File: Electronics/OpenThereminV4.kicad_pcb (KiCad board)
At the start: 2 copper layers, 50.5 x 127.5 mm, 102 parts, among them J1 USB_C_Receptacle, J2 Conn_02x03_Odd_Even, P1 10k, P10 BUTTON, P11 A3_PAD, P12 A2_PAD, P13 A1_PAD, P14 A0_PAD, P15 CV2, P16 GND, P2 10k, P3 10k, P4 10k, P5 RXD, P6 audio, P7 CV1, P8 VCC, P9 GND, U1 TTP223, U10 FT232RL, U11 LP2985-3.3, U12 MCP4922-E/SL, U2 74HC4060D, U3 74HC4060D, U4 74HC74, U5 HEF4069UBT, U6 MCP4922-E/SL, U7 MCP4922-E/SL, U8 LM358 / MCP6002, U9 ATmega328P-AU, X1 16MHz, X2 7.3721MHz, Y1 MountPad3, Y2 MountPad3, Y3 SJ-3524-SMT-TR, Y7 SJ-3524-SMT-TR

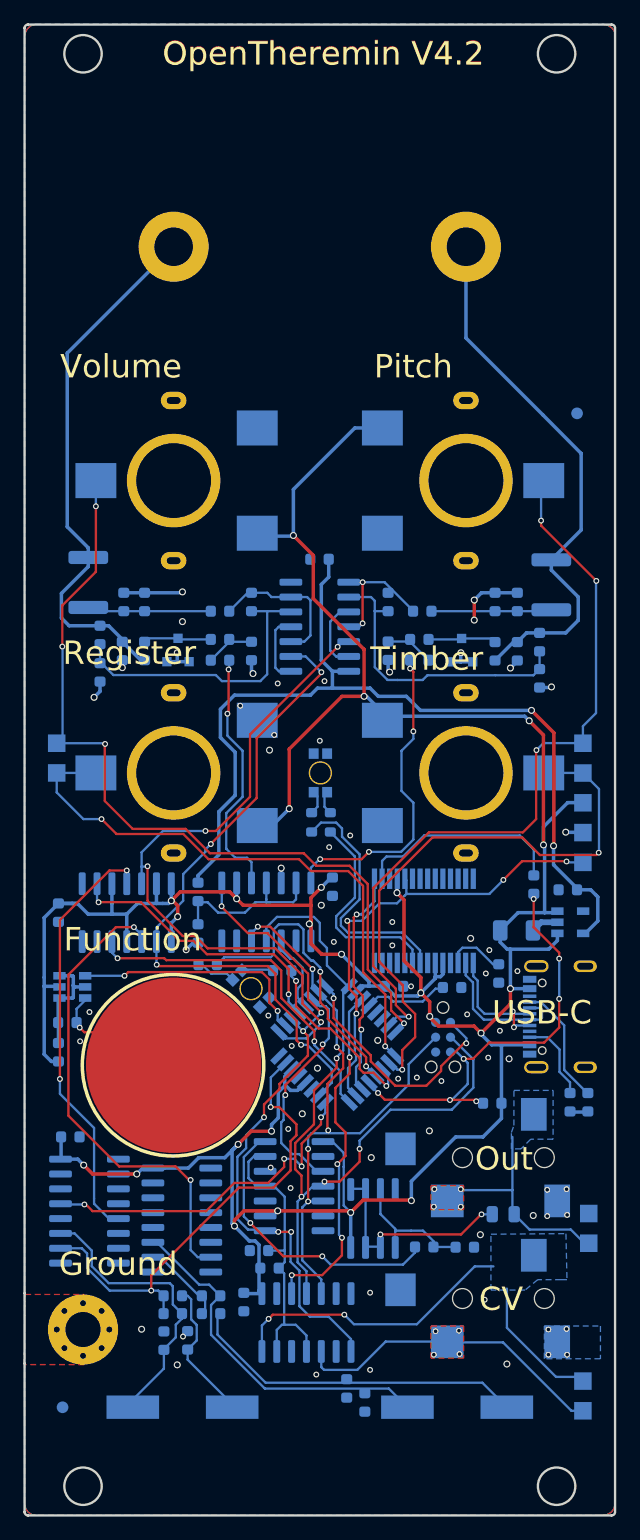
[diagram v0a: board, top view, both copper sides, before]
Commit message: update files
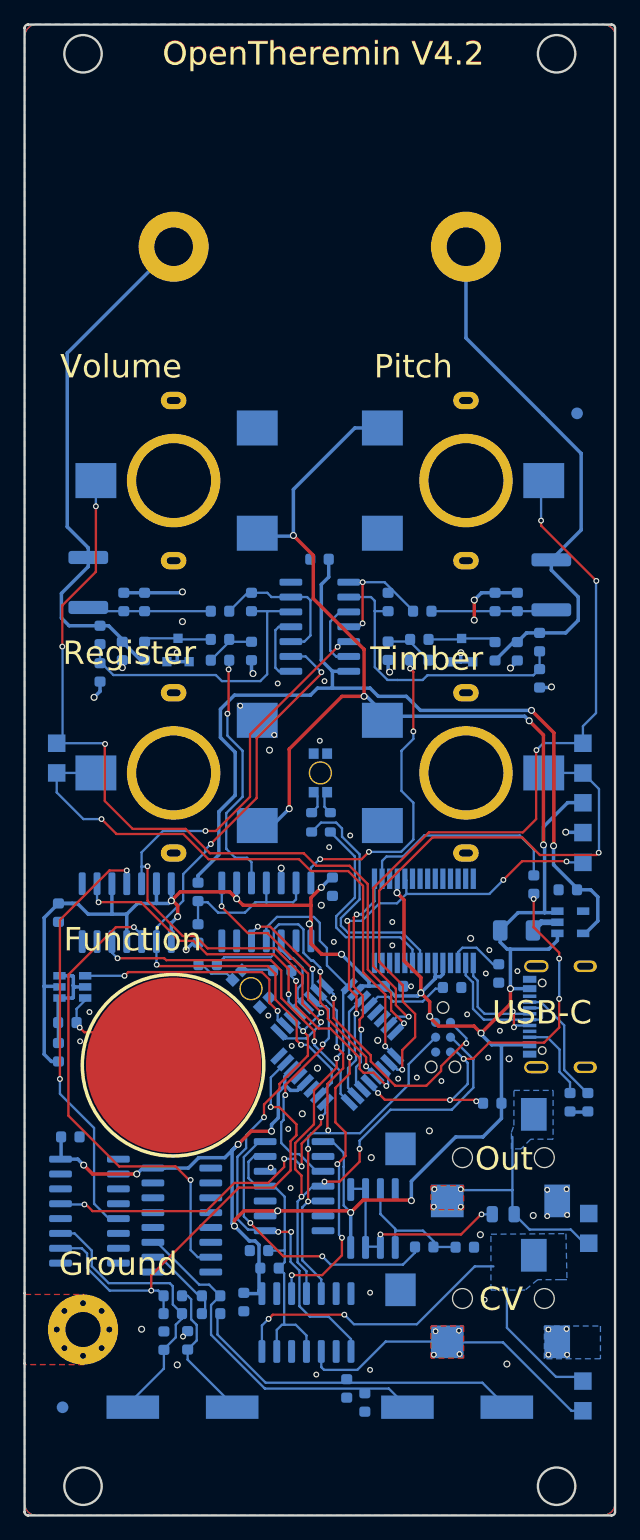
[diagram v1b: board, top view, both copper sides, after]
